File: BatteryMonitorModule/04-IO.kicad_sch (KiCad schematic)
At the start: 30 parts, among them J10 J_DISP_SPI, J11 J_UART, J12 J_EXP_B, J13 J_EXP_A, J5 J_FAN, J6 J_FAN_SEL, J7 J_NFC, J8 J_PANEL, J9 J_DISP_I2C, Q5 2N7002

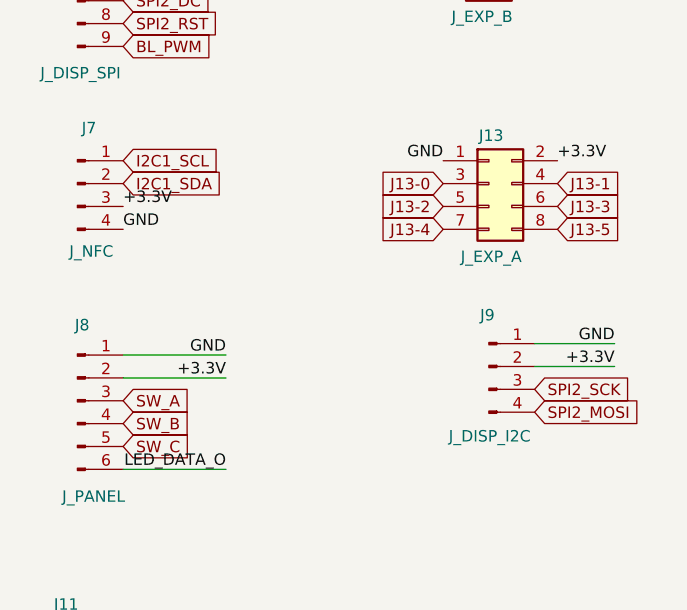
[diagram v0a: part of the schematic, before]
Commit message: routed
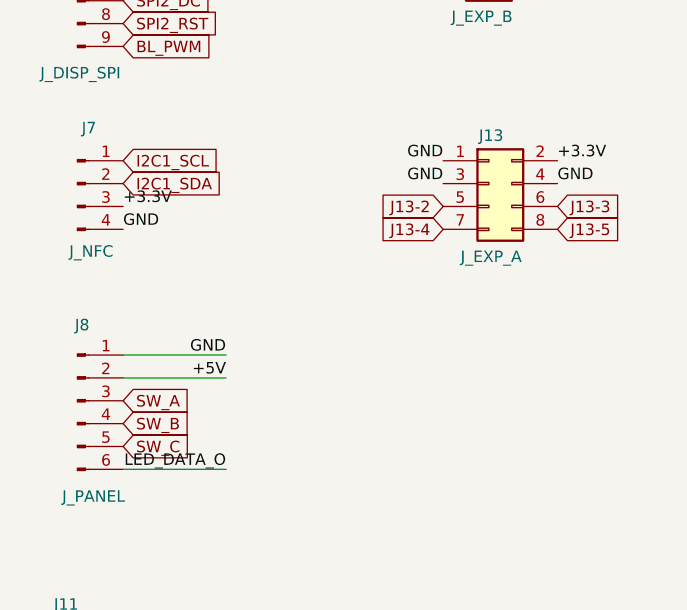
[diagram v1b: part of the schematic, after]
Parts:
- removed J9: J_DISP_I2C, Connector_JST:JST_XH_B4B-XH-A_1x04_P2.50mm_Vertical, symbol Connector:Conn_01x04_Pin
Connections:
- net J13-0 is gone; now on net GND: J13.3 (Pin_3)
- net J13-1 is gone; now on net GND: J13.4 (Pin_4)
- net +3.3V: no longer J8.2 (Pin_2)
- net +5V: now also J8.2 (Pin_2)
